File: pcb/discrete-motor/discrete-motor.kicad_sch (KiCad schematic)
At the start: 28 parts, among them J1 ScrewTerminal, U1 PinHeader8, U2 PinHeader8

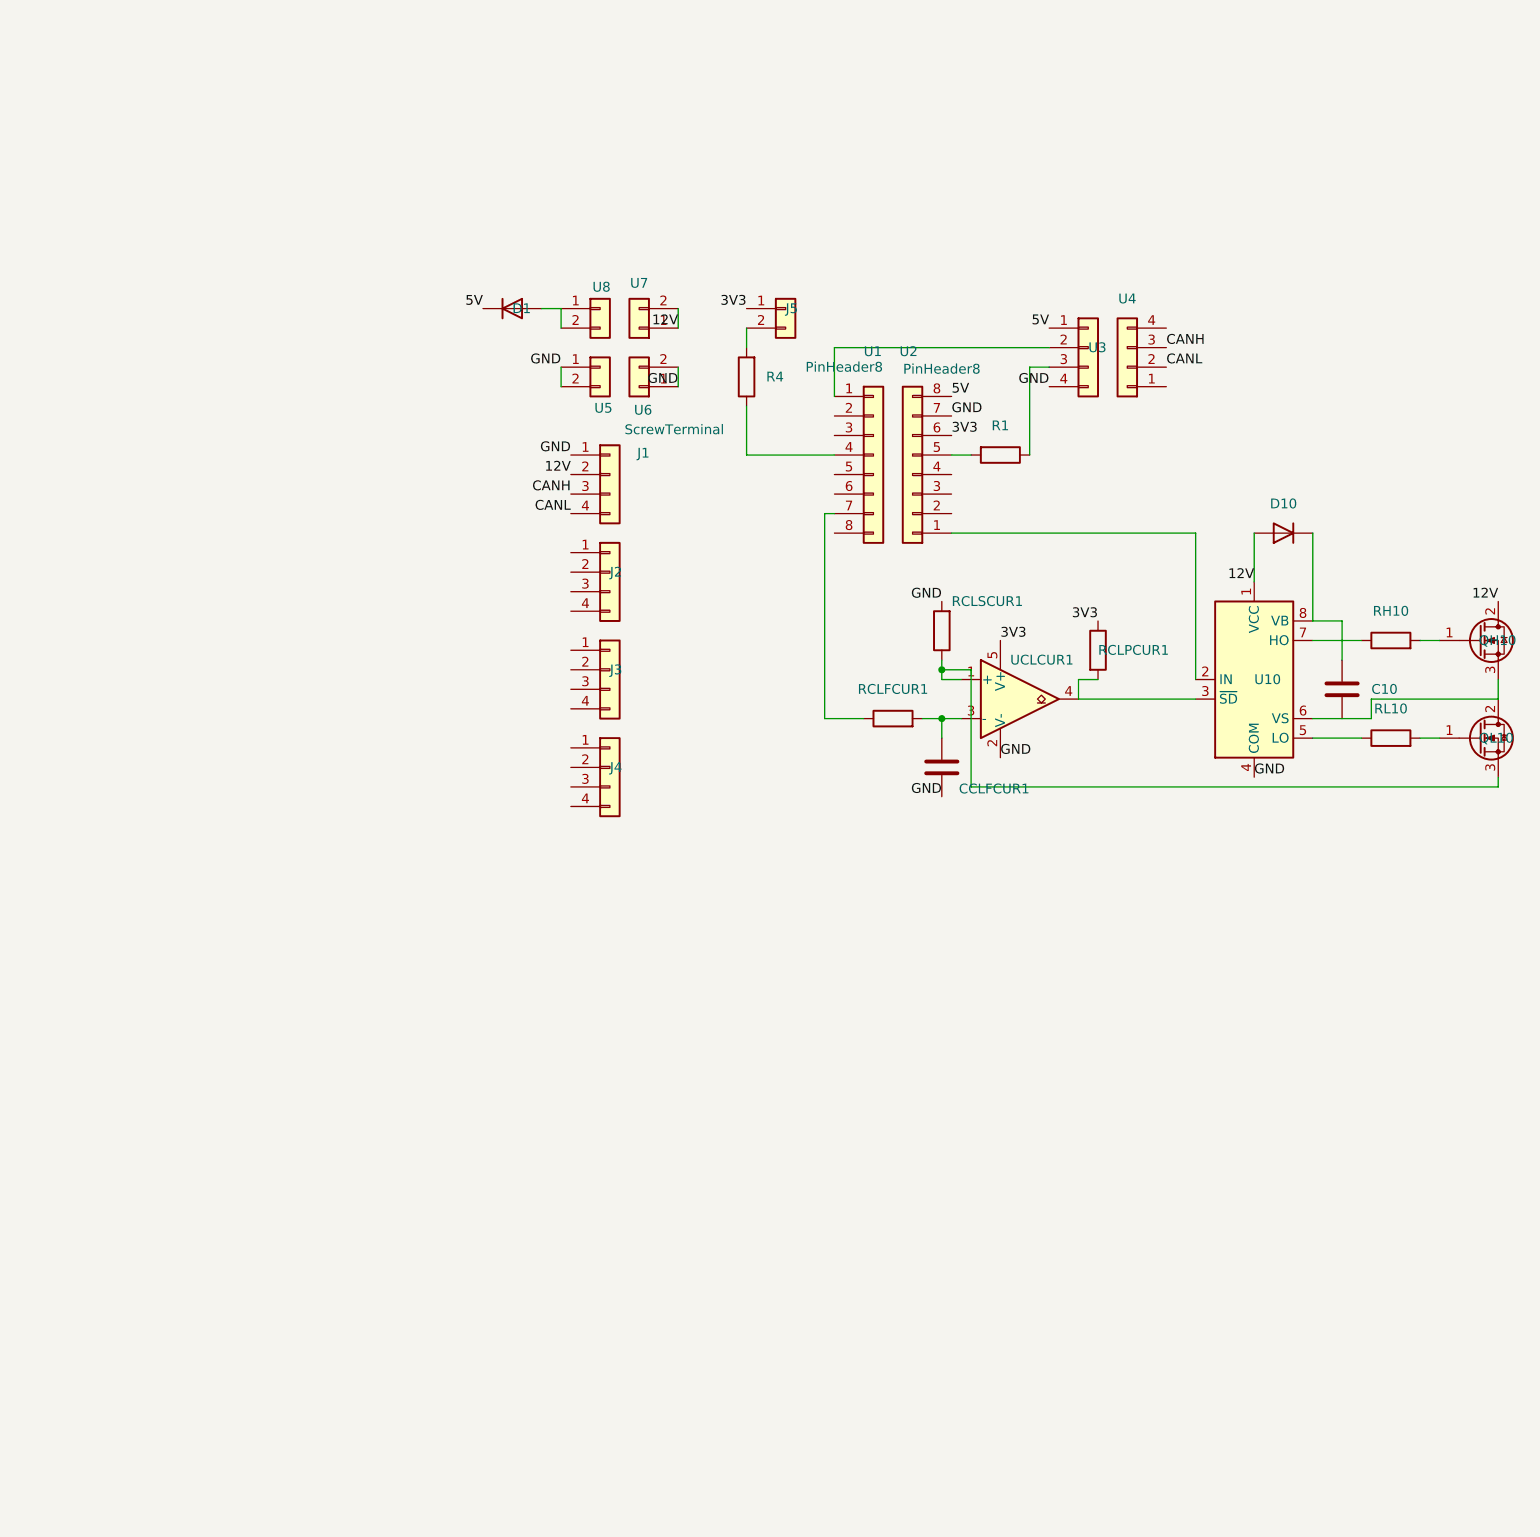
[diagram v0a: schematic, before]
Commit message: wip
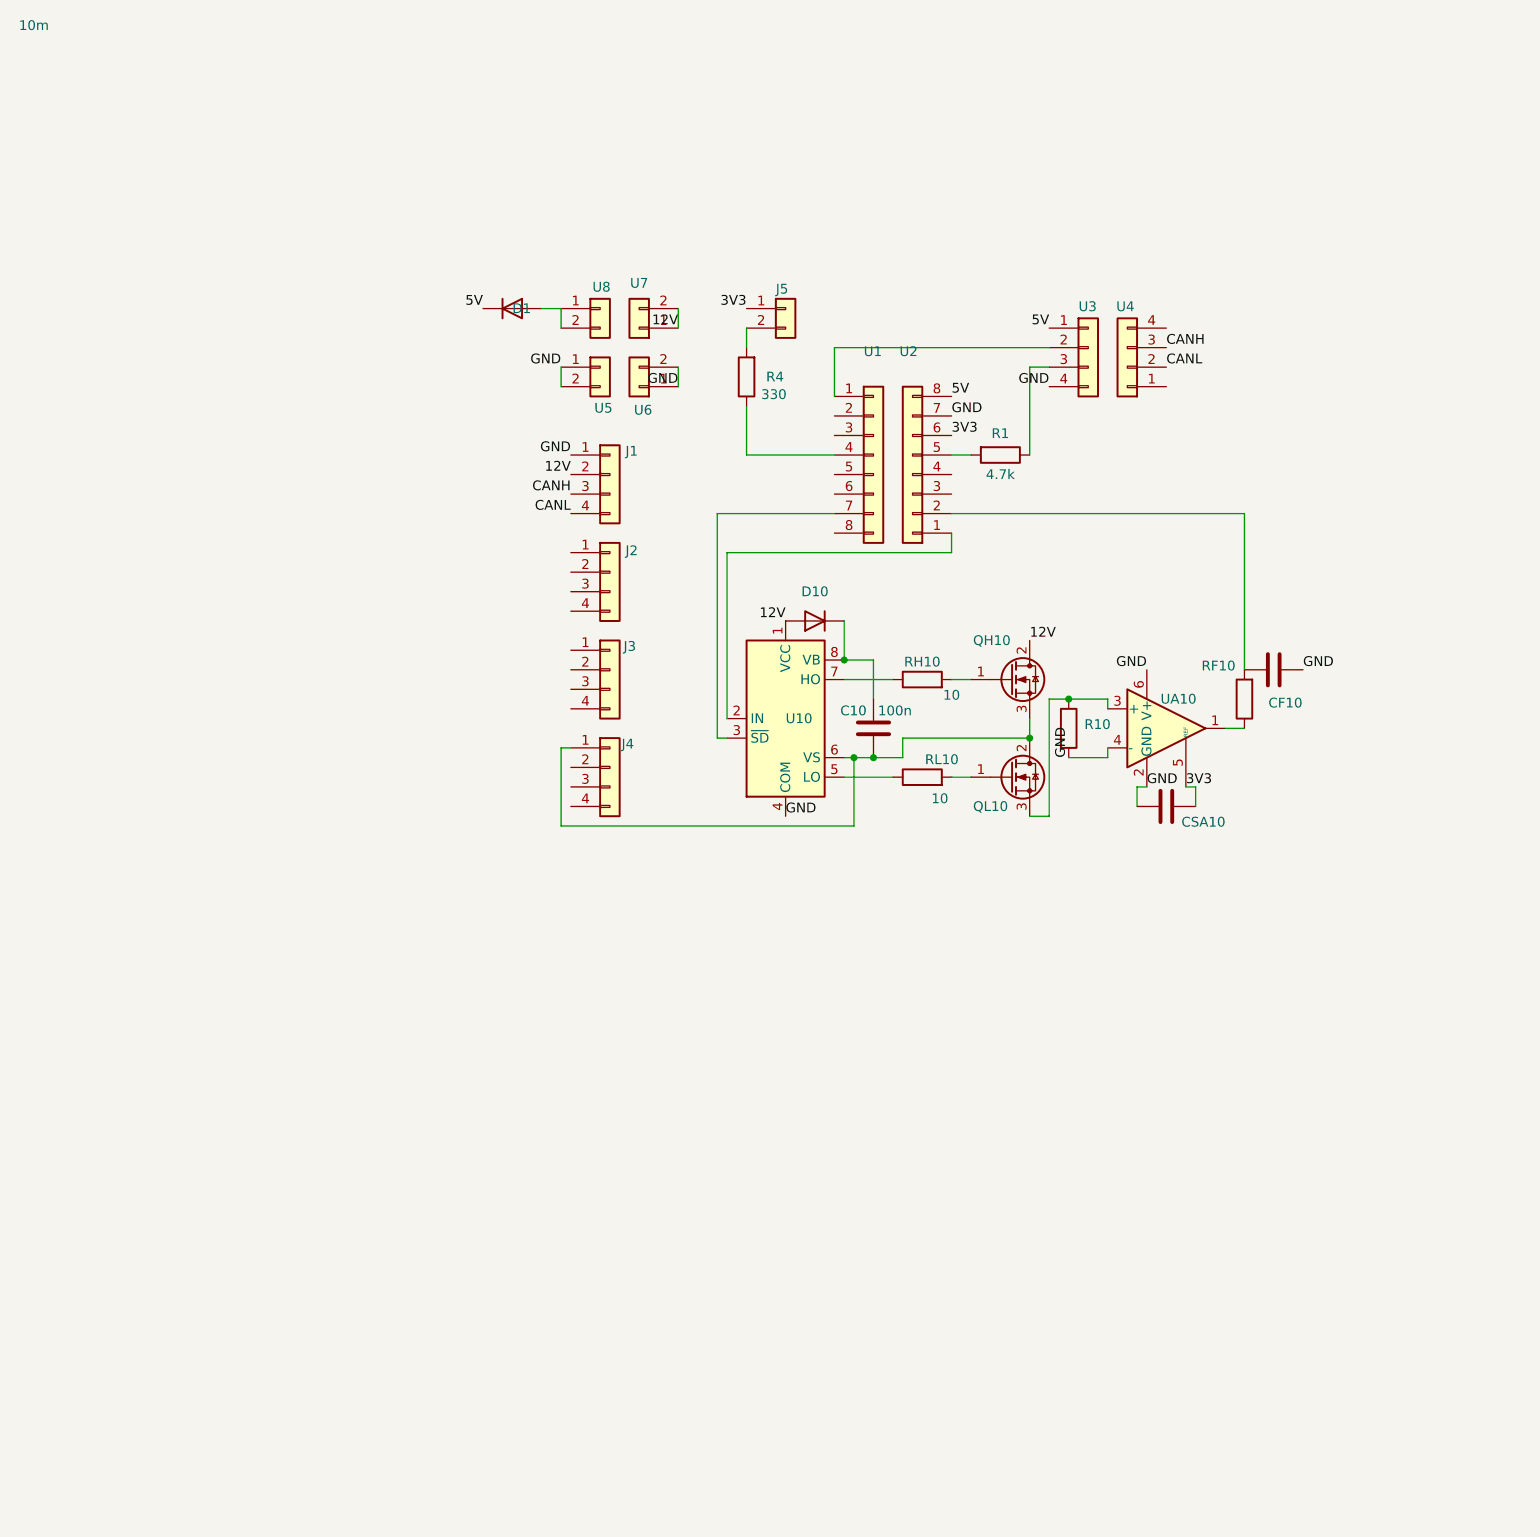
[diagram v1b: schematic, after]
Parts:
- removed CCLFCUR1: (no value), Capacitor_SMD:C_0603_1608Metric, symbol Device:C
- removed RCLFCUR1, RCLPCUR1, RCLSCUR1: (no value), Resistor_SMD:R_0603_1608Metric, symbol Device:R
- removed UCLCUR1: (no value), Package_SO:SOIC-5, symbol Comparator:LMV331
- added CF10, CSA10: 100n, Capacitor_SMD:C_0603_1608Metric, symbol Device:C
- added R10: 10m, Resistor_SMD:R_1206_3216Metric, symbol Device:R
- added RF10: 1k, Resistor_SMD:R_0603_1608Metric, symbol Device:R
- added UA10: (no value), Package_TO_SOT_SMD:SOT-23-6, symbol Amplifier_Current:INA181
- C10: value (none) -> 100n
- J1: value ScrewTerminal -> (none)
- QH10, QL10: footprint Package_TO_SOT_THT:TO-263-2 -> fixme!!!
- R1: value (none) -> 4.7k
- R4: value (none) -> 330
- RH10, RL10: value (none) -> 10
- U1, U2: value PinHeader8 -> (none)
- U3, U4: value ~ -> (none)
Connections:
- net 3V3: now also CSA10.1, UA10.5 (REF)
- net GND: now also CF10.2, CSA10.2, R10.2, UA10.2 (GND), UA10.4 (-), UA10.6 (V+)
- net at U10.3 (~{SD}): now also U1.7 (Pin_7)
- net at U2.2 (Pin_2): now also CF10.1, RF10.2
- net at J4.1 (Pin_1): now also C10.2, QH10.3 (S), QL10.2 (D), U10.6 (VS)
- net at QL10.3 (S): now also R10.1, UA10.3 (+)
- new net: RF10.1, UA10.1
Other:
- moved on the sheet: C10, D10, QH10, QL10, RH10, RL10, U10

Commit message: wip
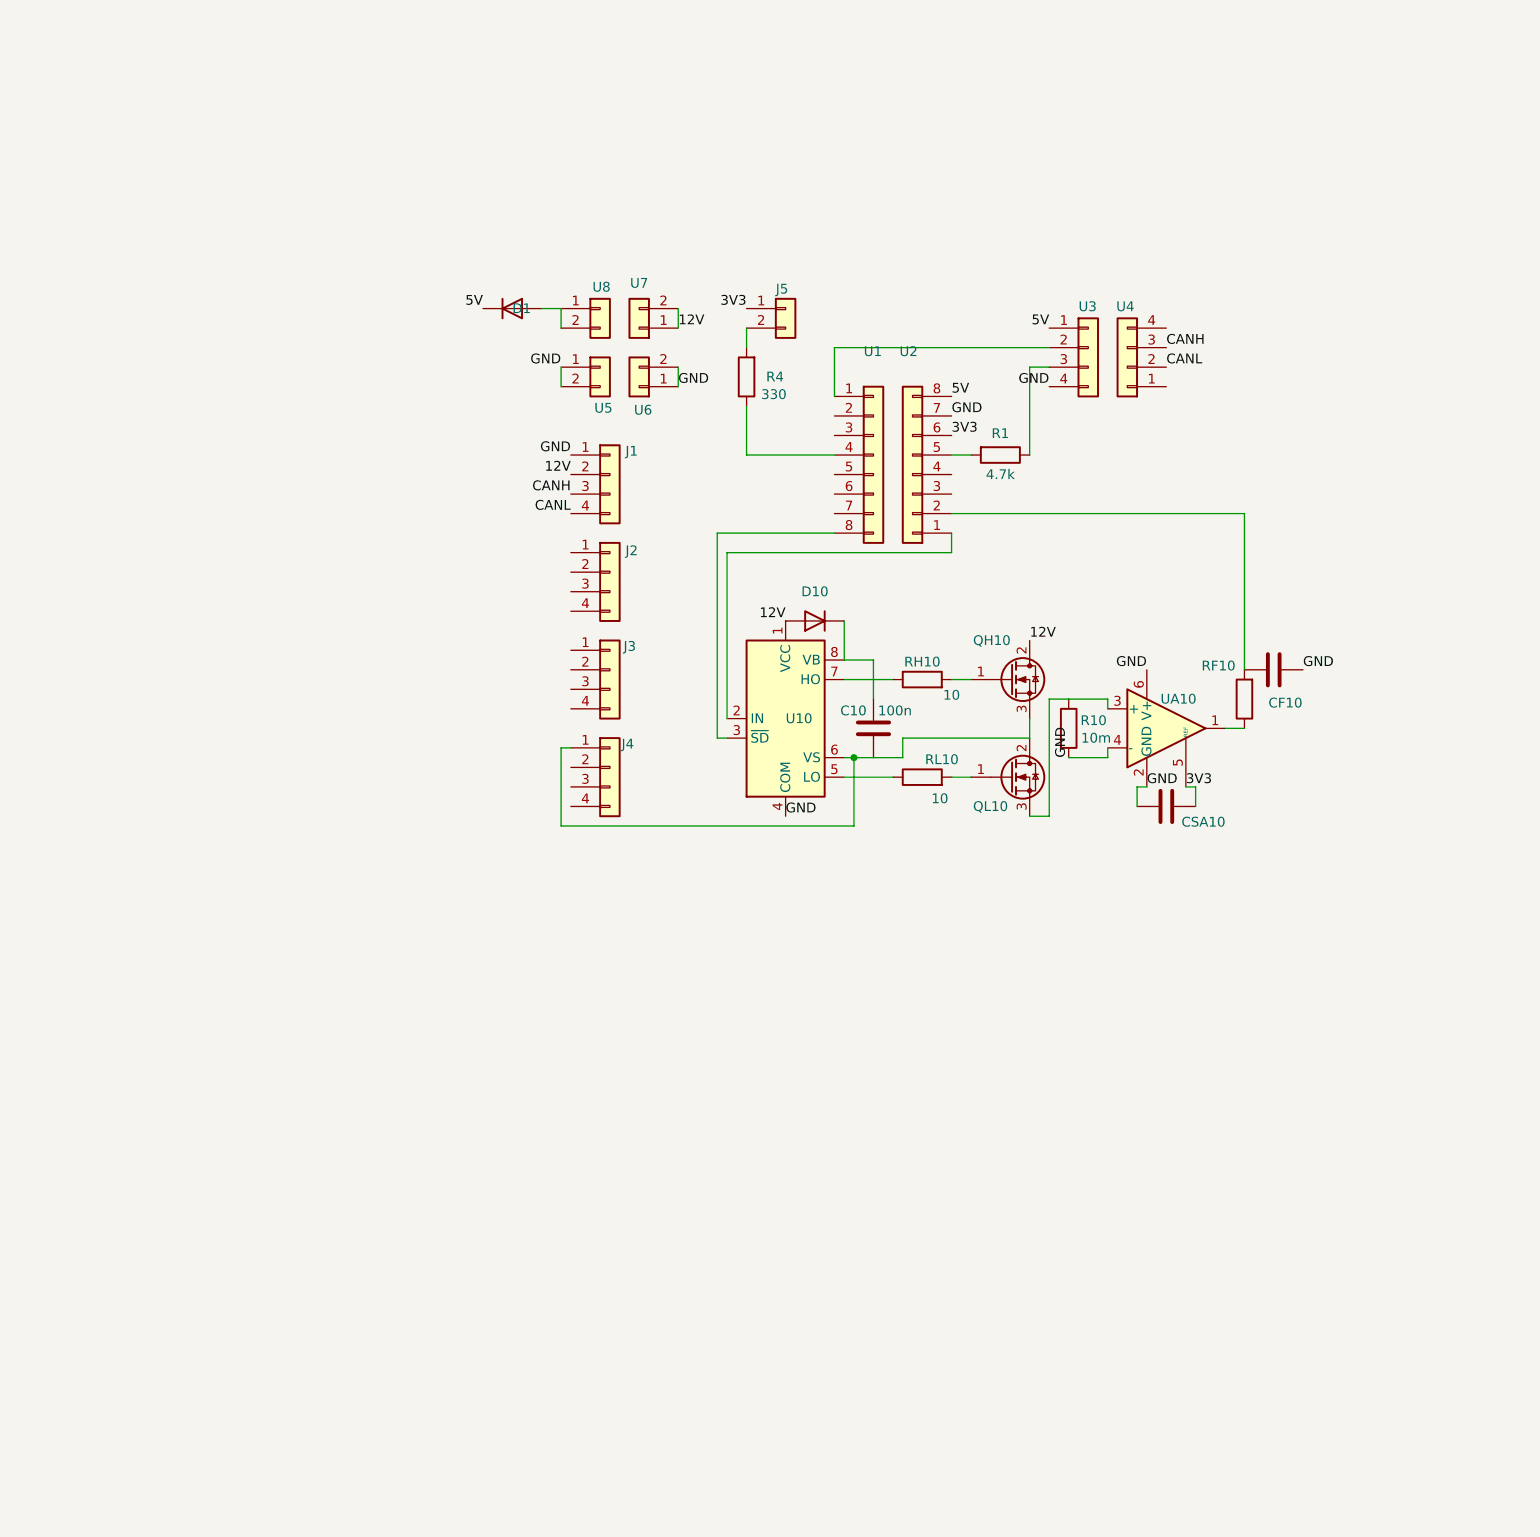
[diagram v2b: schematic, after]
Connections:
- net at U1.7 (Pin_7): no longer U10.3 (~{SD})
- net at U1.8 (Pin_8): now also U10.3 (~{SD})
